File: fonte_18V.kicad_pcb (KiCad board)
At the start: 2 copper layers, 100 x 52 mm, 35 parts, among them J1 MSTBA, J2 MSTBA, J3 RJ45_Shielded, J4 RJ45_Shielded, Q1 Si2308CDS, U1 LMR16030

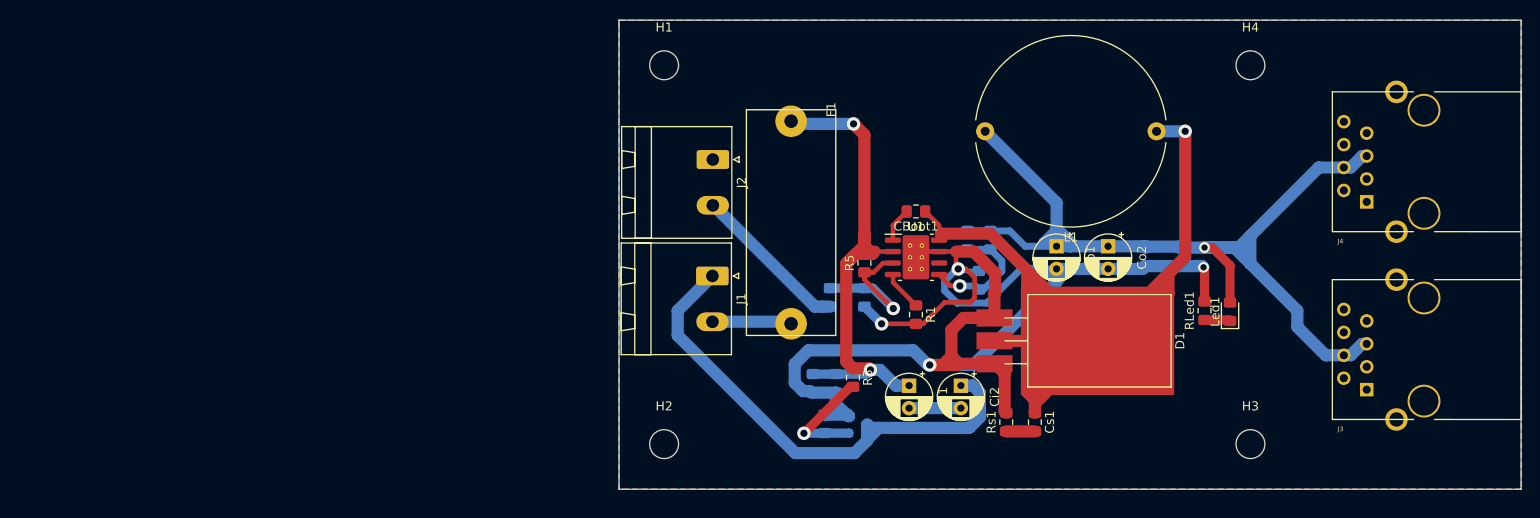
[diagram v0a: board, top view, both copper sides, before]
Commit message: atualizado
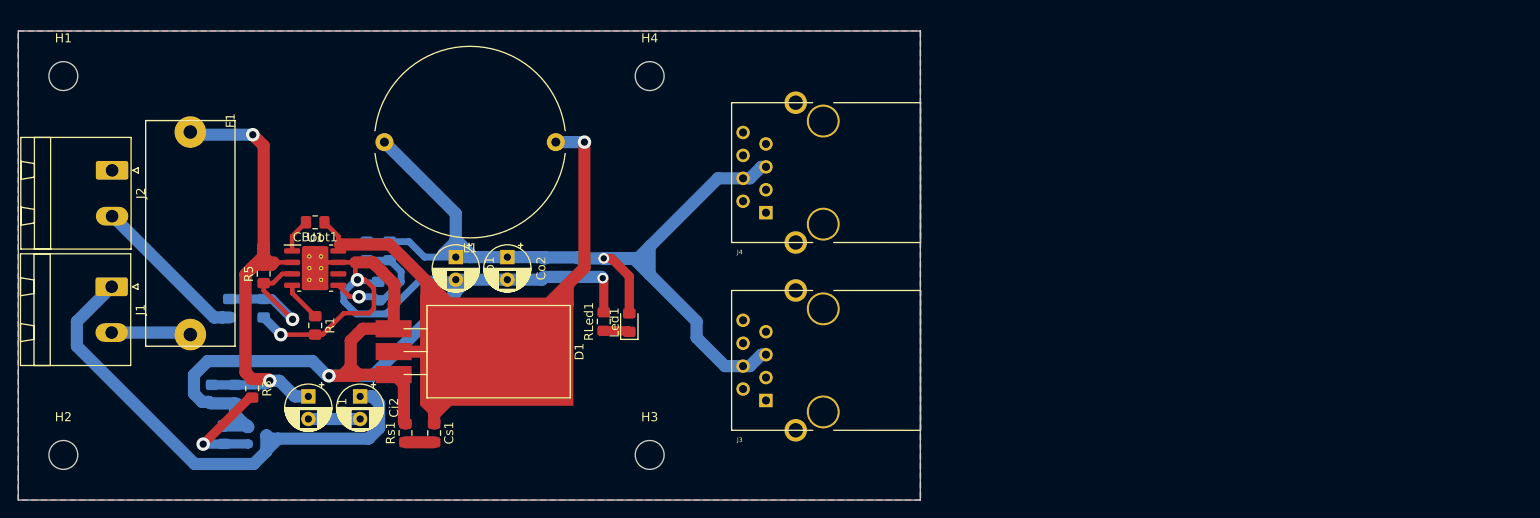
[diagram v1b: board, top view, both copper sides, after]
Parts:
- moved Cff1 66.6 mm to (63.6, 160.6)
- moved Ci2 66.6 mm to (60.3, 176.7)
- moved Co3 66.6 mm to (84.6, 162.4)
- moved Co4 66.6 mm to (80.8, 162.4)
- moved D1 66.6 mm to (64.0, 169.2)
- moved J2 66.6 mm to (32.8, 151.7)
- moved L1 66.6 mm to (82.0, 148.5)
- moved Led1 66.6 mm to (90.1, 168.5)
- moved Rfbt2 66.6 mm to (61.0, 160.6)
- moved Rs1 66.6 mm to (65.3, 180.8)
- moved CBoot1 66.6 mm to (55.3, 157.4)
- moved Ci1 66.6 mm to (54.6, 176.7)
- moved Cin2 66.6 mm to (46.4, 176.5)
- moved Cin3 66.6 mm to (43.9, 176.5)
- moved Co1 66.6 mm to (70.9, 161.3)
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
